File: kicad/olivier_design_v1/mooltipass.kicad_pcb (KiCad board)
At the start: 4 copper layers, 65 parts, among them CON2 CON_10118194-0001LF, P1 CONN_8, P2 CONN_6, P3 CONN_10, P4 CONN_8, P5 CONN_1, P6 CONN_1, P7 CONN_1, P8 CONN_1, Q1 MOS_P, Q2 MOS_N, Q3 MOS_P, Q4 MOS_N, U1 CON_SFV30R-2STE1HLF, U2 CON_7312P0225A13LF, U3 IP4234CZ6,125, U4 ATMEGA32U4_QFN, U5 ST662ACD, U6 AT45DB011D-SSH, U7 CON_STACK_9, X1 16MHz

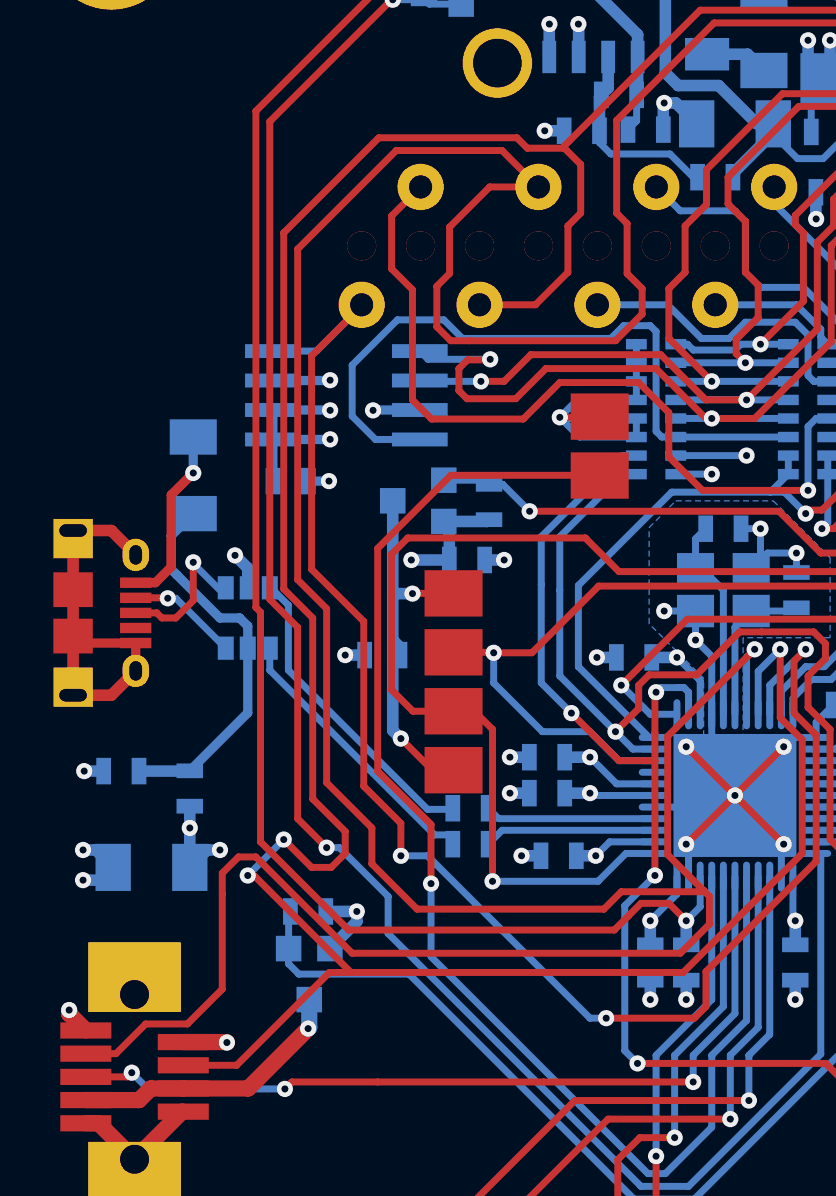
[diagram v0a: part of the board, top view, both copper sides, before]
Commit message: updating bottom PCB
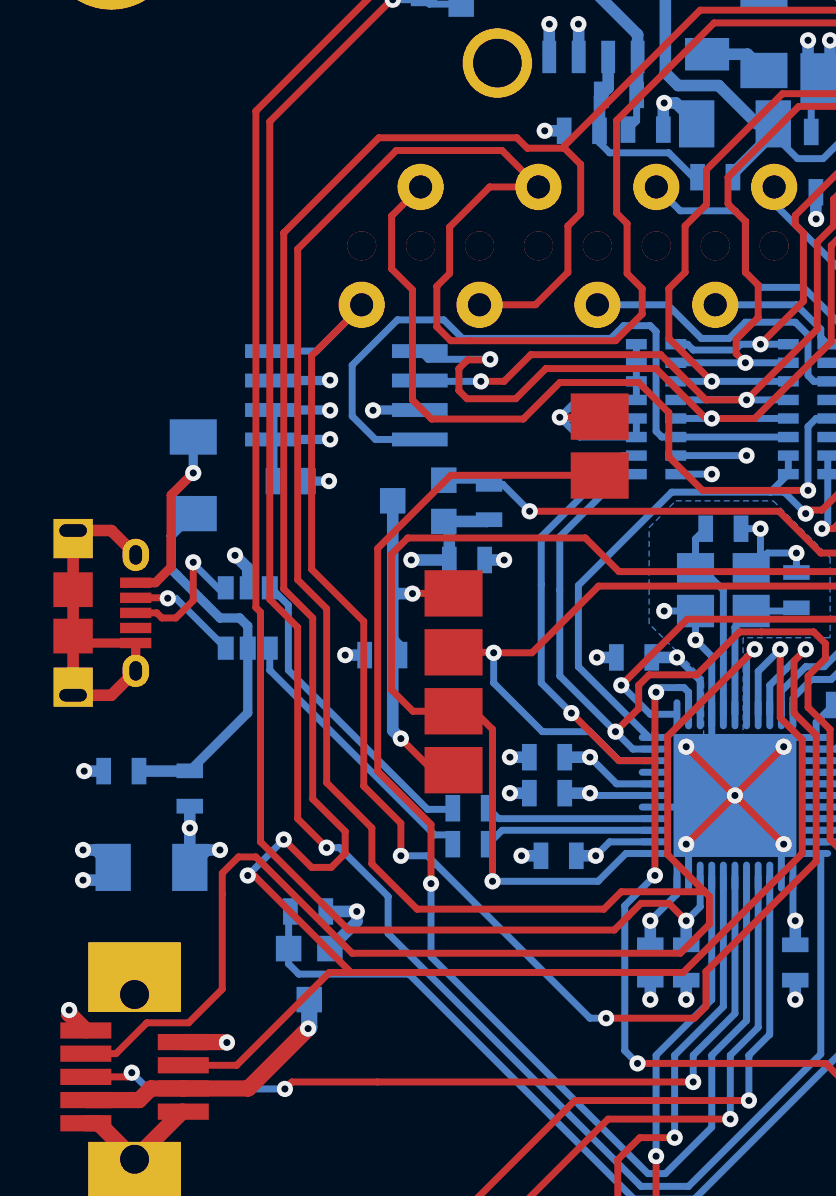
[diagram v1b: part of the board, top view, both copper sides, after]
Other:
- board text added: "Mooltipass by M.Stephan Licensed under CERN OHL V1.2"
- board text removed: "Mooltipass M.Stephan / limpkin For Olivier's design Licensed under CERN OHL V1.2"
